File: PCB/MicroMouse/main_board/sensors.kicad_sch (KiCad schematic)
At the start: 5 parts, among them J4 Conn_01x06, J5 Conn_01x06, J6 Conn_01x06, J7 Conn_01x06, J8 Conn_01x06

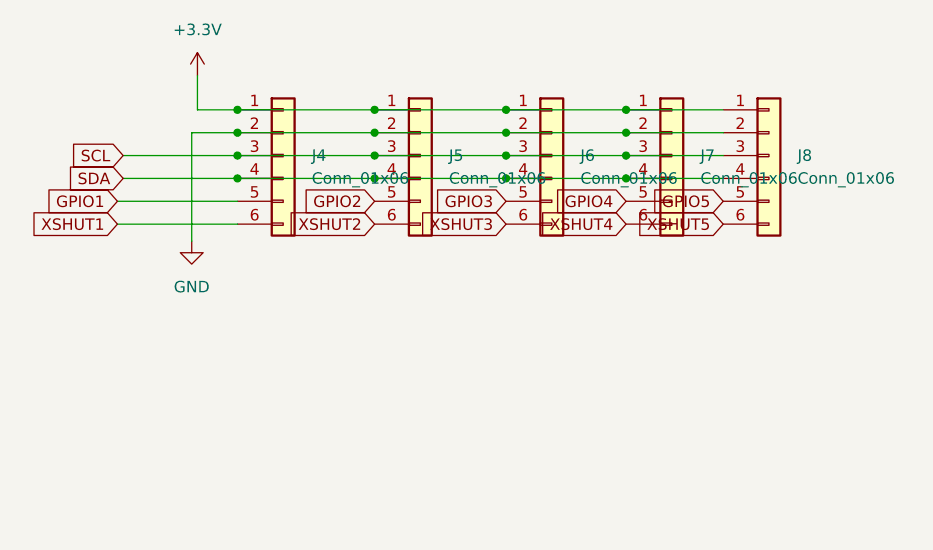
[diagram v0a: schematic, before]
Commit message: PCB prototype
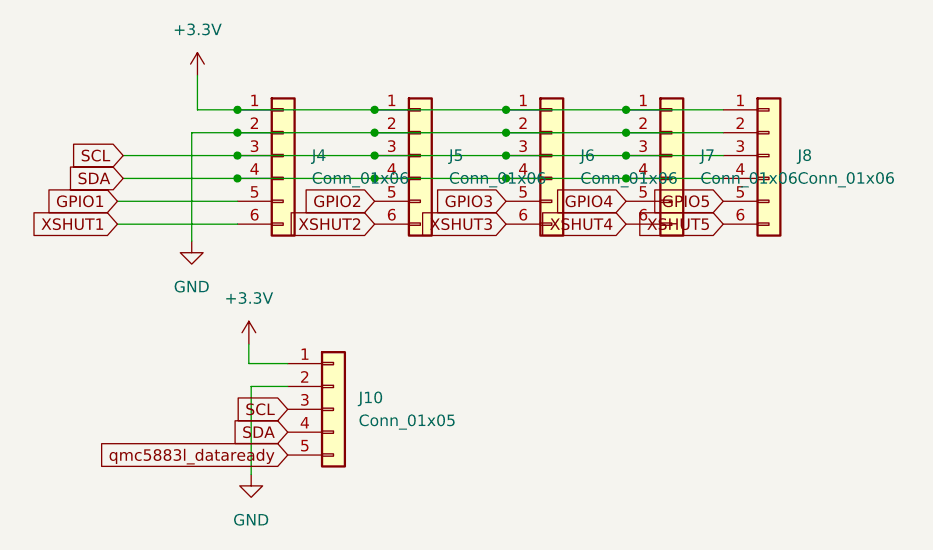
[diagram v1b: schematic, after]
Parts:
- added J10: Conn_01x05, Connector_PinSocket_2.54mm:PinSocket_1x05_P2.54mm_Vertical, symbol Connector_Generic:Conn_01x05
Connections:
- net +3V3: now also J10.1 (Pin_1)
- net GND: now also J10.2 (Pin_2)
- net SCL: now also J10.3 (Pin_3)
- net SDA: now also J10.4 (Pin_4)
- new net qmc5883l_dataready: J10.5 (Pin_5)
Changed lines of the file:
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@@
+    (stroke (width 0) (type default))
+  )
+  (wire (pts (xy 47.244 66.548) (xy 47.244 56.769))
     (stroke (width 0) (type default))
   )
@@
     (stroke (width 0) (type default))
   )
+  (wire (pts (xy 46.99 52.07) (xy 46.99 54.229))
+    (stroke (width 0) (type default))
+  )
   (wire (pts (xy 75.565 26.035) (xy 88.9 26.035))
     (stroke (width 0) (type default))
   )
+  (wire (pts (xy 47.244 56.769) (xy 51.308 56.769))
+    (stroke (width 0) (type default))
+  )
+  (wire (pts (xy 46.99 54.229) (xy 51.308 54.229))
+    (stroke (width 0) (type default))
+  )
   (wire (pts (xy 45.72 31.115) (xy 60.96 31.115))
     (stroke (width 0) (type default))
@@
     )
   )
+  (global_label "SDA" (shape input) (at 51.308 61.849 180) (fields_autoplaced)
+    (effects (font (size 1.27 1.27)) (justify right))
+    (property "Intersheetrefs" "${INTERSHEET_REFS}" (at 44.7547 61.849 0)
+      (effects (font (size 1.27 1.27)) (justify right) hide)
+    )
+  )
   (global_label "XSHUT2" (shape input) (at 60.96 38.735 180) (fields_autoplaced)
     (effects (font (size 1.27 1.27)) (justify right))
@@
     (effects (font (size 1.27 1.27)) (justify right))
     (property "Intersheetrefs" "${INTERSHEET_REFS}" (at 26.4667 33.655 0)
+      (effects (font (size 1.27 1.27)) (justify right) hide)
+    )
+  )
+  (global_label "qmc5883l_dataready" (shape input) (at 51.308 64.389 180) (fields_autoplaced)
+    (effects (font (size 1.27 1.27)) (justify right))
+    (property "Intersheetrefs" "${INTERSHEET_REFS}" (at 28.608 64.389 0)
+      (effects (font (size 1.27 1.27)) (justify right) hide)
+    )
+  )
+  (global_label "SCL" (shape input) (at 51.308 59.309 180) (fields_autoplaced)
+    (effects (font (size 1.27 1.27)) (justify right))
+    (property "Intersheetrefs" "${INTERSHEET_REFS}" (at 44.8152 59.309 0)
       (effects (font (size 1.27 1.27)) (justify right) hide)
     )
@@
     )
   )
+  (symbol (lib_id "power:+3.3V") (at 46.99 52.07 0) (unit 1)
+    (in_bom yes) (on_board yes) (dnp no) (fields_autoplaced)
+    (property "Reference" "#PWR039" (at 46.99 55.88 0)
+      (effects (font (size 1.27 1.27)) hide)
+    )
+    (property "Value" "+3.3V" (at 46.99 46.99 0)
+      (effects (font (size 1.27 1.27)))
+    )
+    (property "Footprint" "" (at 46.99 52.07 0)
+      (effects (font (size 1.27 1.27)) hide)
+    )
+    (property "Datasheet" "" (at 46.99 52.07 0)
+      (effects (font (size 1.27 1.27)) hide)
+    )
+    (pin "1")
+    (instances
+      (project "main_board"
+        (path "/3863100a-f026-49db-8424-2d27c05016cc/e041bfaf-2492-4cbf-be74-a40fc3304146"
+          (reference "#PWR039") (unit 1)
+        )
+      )
+    )
+  )
   (symbol (lib_id "Connector_Generic:Conn_01x06") (at 66.04 31.115 0) (unit 1)
     (in_bom yes) (on_board yes) (dnp no) (fields_autoplaced)
@@
       (effects (font (size 1.27 1.27)) hide)
     )
-    (property "Datasheet" "~" (at 66.04 31.115 0)
+    (property "Datasheet" "https://www.laskakit.cz/laserovy-senzor-vzdalenosti-vl53l1x-i2c/" (at 66.04 31.115 0)
       (effects (font (size 1.27 1.27)) hide)
     )
@@
         (path "/3863100a-f026-49db-8424-2d27c05016cc/e041bfaf-2492-4cbf-be74-a40fc3304146"
           (reference "J5") (unit 1)
+        )
+      )
+    )
+  )
+  (symbol (lib_id "Connector_Generic:Conn_01x05") (at 56.388 59.309 0) (unit 1)
+    (in_bom yes) (on_board yes) (dnp no) (fields_autoplaced)
+    (property "Reference" "J10" (at 59.182 58.039 0)
+      (effects (font (size 1.27 1.27)) (justify left))
+    )
+    (property "Value" "Conn_01x05" (at 59.182 60.579 0)
+      (effects (font (size 1.27 1.27)) (justify left))
+    )
+    (property "Footprint" "Connector_PinSocket_2.54mm:PinSocket_1x05_P2.54mm_Vertical" (at 56.388 59.309 0)
+      (effects (font (size 1.27 1.27)) hide)
+    )
+    (property "Datasheet" "https://www.laskakit.cz/arduino-kompas-qmc5883l/?currency=eur&gad_source=4" (at 56.388 59.309 0)
+      (effects (font (size 1.27 1.27)) hide)
+    )
+    (pin "3")
+    (pin "4")
+    (pin "5")
+    (pin "1")
+    (pin "2")
+    (instances
+      (project "main_board"
+        (path "/3863100a-f026-49db-8424-2d27c05016cc/e041bfaf-2492-4cbf-be74-a40fc3304146"
+          (reference "J10") (unit 1)
         )
       )
@@
       (effects (font (size 1.27 1.27)) hide)
     )
-    (property "Datasheet" "~" (at 104.775 31.115 0)
+    (property "Datasheet" "https://www.laskakit.cz/laserovy-senzor-vzdalenosti-vl53l1x-i2c/" (at 104.775 31.115 0)
       (effects (font (size 1.27 1.27)) hide)
     )
@@
     )
   )
+  (symbol (lib_id "power:GND") (at 47.244 66.548 0) (unit 1)
+    (in_bom yes) (on_board yes) (dnp no) (fields_autoplaced)
+    (property "Reference" "#PWR040" (at 47.244 72.898 0)
+      (effects (font (size 1.27 1.27)) hide)
+    )
+    (property "Value" "GND" (at 47.244 71.628 0)
+      (effects (font (size 1.27 1.27)))
+    )
+    (property "Footprint" "" (at 47.244 66.548 0)
+      (effects (font (size 1.27 1.27)) hide)
+    )
+    (property "Datasheet" "" (at 47.244 66.548 0)
+      (effects (font (size 1.27 1.27)) hide)
+    )
+    (pin "1")
+    (instances
+      (project "main_board"
+        (path "/3863100a-f026-49db-8424-2d27c05016cc/e041bfaf-2492-4cbf-be74-a40fc3304146"
+          (reference "#PWR040") (unit 1)
+        )
+      )
+    )
+  )
   (symbol (lib_id "Connector_Generic:Conn_01x06") (at 80.645 31.115 0) (unit 1)
     (in_bom yes) (on_board yes) (dnp no) (fields_autoplaced)
@@
       (effects (font (size 1.27 1.27)) hide)
     )
-    (property "Datasheet" "~" (at 80.645 31.115 0)
+    (property "Datasheet" "https://www.laskakit.cz/laserovy-senzor-vzdalenosti-vl53l1x-i2c/" (at 80.645 31.115 0)
       (effects (font (size 1.27 1.27)) hide)
     )
@@
       (effects (font (size 1.27 1.27)) hide)
     )
-    (property "Datasheet" "~" (at 93.98 31.115 0)
+    (property "Datasheet" "https://www.laskakit.cz/laserovy-senzor-vzdalenosti-vl53l1x-i2c/" (at 93.98 31.115 0)
       (effects (font (size 1.27 1.27)) hide)
     )
@@
       (effects (font (size 1.27 1.27)) hide)
     )
-    (property "Datasheet" "~" (at 50.8 31.115 0)
-      (effects (font (size 1.27 1.27)) hide)
-    )
+    (property "Datasheet" "https://www.laskakit.cz/laserovy-senzor-vzdalenosti-vl53l1x-i2c/" (at 50.8 31.115 0)
+      (effects (font (size 1.27 1.27)) hide)
+    )

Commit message: some changes on PCB after consultations with Mr. micromouse FEI
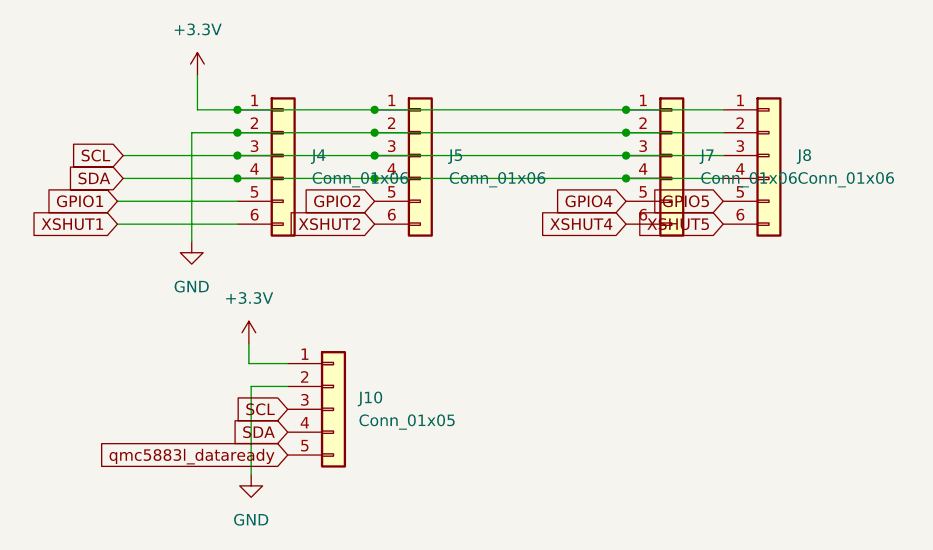
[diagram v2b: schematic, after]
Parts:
- removed J6: Conn_01x06, Connector_PinSocket_2.54mm:PinSocket_1x06_P2.54mm_Vertical, symbol Connector_Generic:Conn_01x06
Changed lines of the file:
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@@
   (junction (at 45.72 26.035) (diameter 0) (color 0 0 0 0)
   )
-  (junction (at 75.565 31.115) (diameter 0) (color 0 0 0 0)
-  )
   (junction (at 45.72 31.115) (diameter 0) (color 0 0 0 0)
   )
@@
   (junction (at 60.96 26.035) (diameter 0) (color 0 0 0 0)
   )
-  (junction (at 75.565 33.655) (diameter 0) (color 0 0 0 0)
-  )
   (junction (at 60.96 31.115) (diameter 0) (color 0 0 0 0)
   )
@@
   (junction (at 88.9 33.655) (diameter 0) (color 0 0 0 0)
   )
-  (junction (at 75.565 28.575) (diameter 0) (color 0 0 0 0)
-  )
-  (junction (at 75.565 26.035) (diameter 0) (color 0 0 0 0)
-  )
   (wire (pts (xy 40.64 28.575) (xy 40.64 40.64))
     (stroke (width 0) (type default))
   )
-  (wire (pts (xy 60.96 28.575) (xy 75.565 28.575))
+  (wire (pts (xy 60.96 28.575) (xy 88.9 28.575))
     (stroke (width 0) (type default))
   )
@@
     (stroke (width 0) (type default))
   )
-  (wire (pts (xy 60.96 33.655) (xy 75.565 33.655))
+  (wire (pts (xy 60.96 33.655) (xy 88.9 33.655))
     (stroke (width 0) (type default))
   )
@@
     (stroke (width 0) (type default))
   )
-  (wire (pts (xy 60.96 31.115) (xy 75.565 31.115))
-    (stroke (width 0) (type default))
-  )
   (wire (pts (xy 88.9 28.575) (xy 99.695 28.575))
     (stroke (width 0) (type default))
@@
     (stroke (width 0) (type default))
   )
-  (wire (pts (xy 75.565 31.115) (xy 88.9 31.115))
+  (wire (pts (xy 60.96 31.115) (xy 88.9 31.115))
     (stroke (width 0) (type default))
   )
@@
     (stroke (width 0) (type default))
   )
-  (wire (pts (xy 75.565 33.655) (xy 88.9 33.655))
-    (stroke (width 0) (type default))
-  )
   (wire (pts (xy 32.385 36.195) (xy 45.72 36.195))
     (stroke (width 0) (type default))
@@
     (stroke (width 0) (type default))
   )
-  (wire (pts (xy 75.565 26.035) (xy 88.9 26.035))
-    (stroke (width 0) (type default))
-  )
   (wire (pts (xy 47.244 56.769) (xy 51.308 56.769))
     (stroke (width 0) (type default))
@@
     (stroke (width 0) (type default))
   )
-  (wire (pts (xy 60.96 26.035) (xy 75.565 26.035))
-    (stroke (width 0) (type default))
-  )
-  (wire (pts (xy 75.565 28.575) (xy 88.9 28.575))
+  (wire (pts (xy 60.96 26.035) (xy 88.9 26.035))
     (stroke (width 0) (type default))
   )
@@
     )
   )
-  (global_label "GPIO3" (shape input) (at 75.565 36.195 180) (fields_autoplaced)
-    (effects (font (size 1.27 1.27)) (justify right))
-    (property "Intersheetrefs" "${INTERSHEET_REFS}" (at 66.895 36.195 0)
-      (effects (font (size 1.27 1.27)) (justify right) hide)
-    )
-  )
   (global_label "XSHUT4" (shape input) (at 88.9 38.735 180) (fields_autoplaced)
     (effects (font (size 1.27 1.27)) (justify right))
@@
     (effects (font (size 1.27 1.27)) (justify right))
     (property "Intersheetrefs" "${INTERSHEET_REFS}" (at 22.1427 38.735 0)
-      (effects (font (size 1.27 1.27)) (justify right) hide)
-    )
-  )
-  (global_label "XSHUT3" (shape input) (at 75.565 38.735 180) (fields_autoplaced)
-    (effects (font (size 1.27 1.27)) (justify right))
-    (property "Intersheetrefs" "${INTERSHEET_REFS}" (at 65.3227 38.735 0)
       (effects (font (size 1.27 1.27)) (justify right) hide)
     )
@@
         )
       )
-    )
-  )
-  (symbol (lib_id "Connector_Generic:Conn_01x06") (at 80.645 31.115 0) (unit 1)
-    (in_bom yes) (on_board yes) (dnp no) (fields_autoplaced)
-    (property "Reference" "J6" (at 83.82 31.115 0)
-      (effects (font (size 1.27 1.27)) (justify left))
-    )
-    (property "Value" "Conn_01x06" (at 83.82 33.655 0)
-      (effects (font (size 1.27 1.27)) (justify left))
-    )
-    (property "Footprint" "Connector_PinSocket_2.54mm:PinSocket_1x06_P2.54mm_Vertical" (at 80.645 31.115 0)
-      (effects (font (size 1.27 1.27)) hide)
-    )
-    (property "Datasheet" "https://www.laskakit.cz/laserovy-senzor-vzdalenosti-vl53l1x-i2c/" (at 80.645 31.115 0)
-      (effects (font (size 1.27 1.27)) hide)
-    )
-    (pin "2")
-    (pin "4")
-    (pin "1")
-    (pin "3")
-    (pin "5")
-    (pin "6")
-    (instances
-      (project "main_board"
-        (path "/3863100a-f026-49db-8424-2d27c05016cc/e041bfaf-2492-4cbf-be74-a40fc3304146"
-          (reference "J6") (unit 1)
-        )
-      )
